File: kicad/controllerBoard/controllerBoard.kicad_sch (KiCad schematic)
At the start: 2 parts, among them J1 Conn_02x20_Top_Bottom, J2 Conn_02x20_Top_Bottom

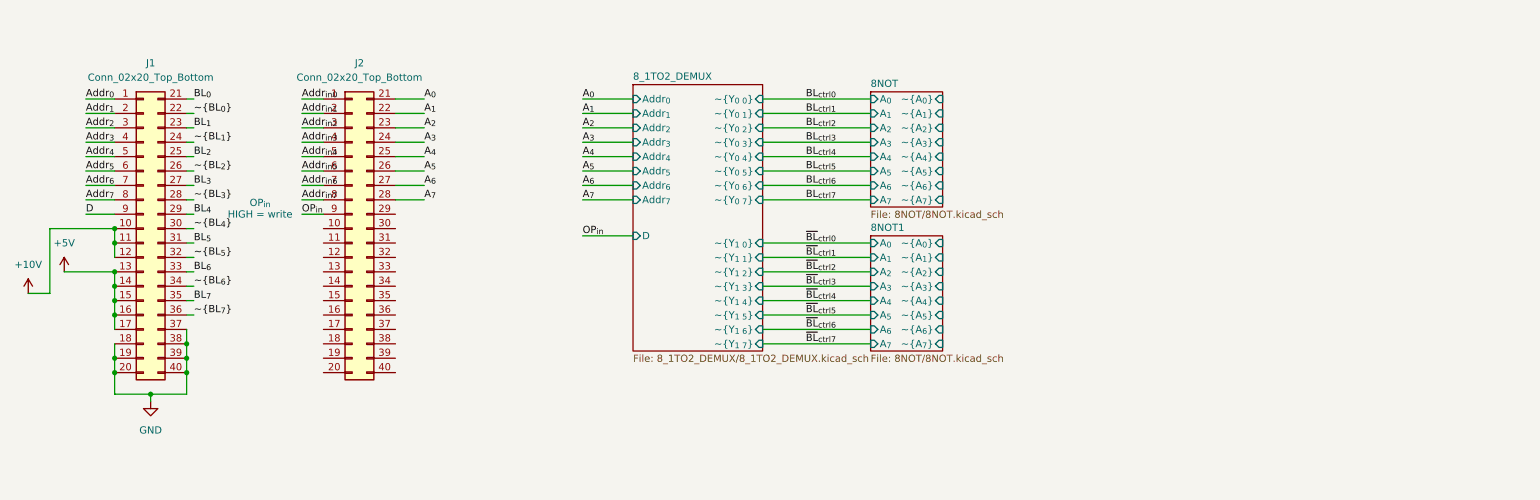
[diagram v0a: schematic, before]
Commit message: demux
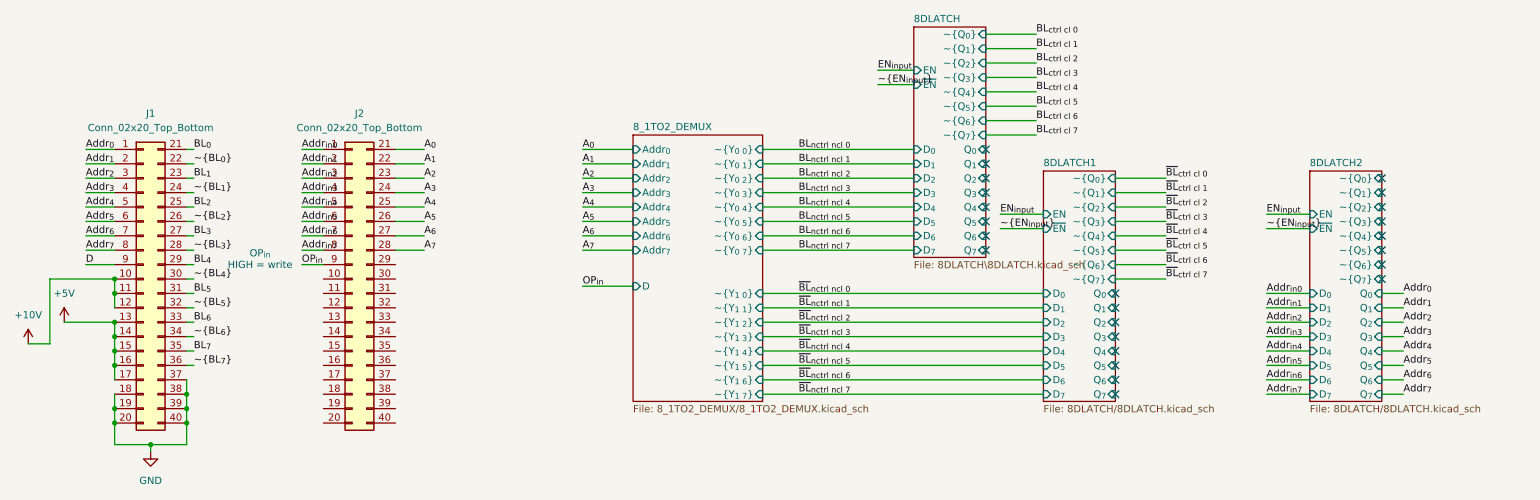
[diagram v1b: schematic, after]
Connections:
- no-connect marks 0 -> 24
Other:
- removed sheet 8NOT
- removed sheet 8NOT1
- added sheet 8DLATCH (8DLATCH\8DLATCH.kicad_sch)
- added sheet 8DLATCH1 (8DLATCH/8DLATCH.kicad_sch)
- added sheet 8DLATCH2 (8DLATCH/8DLATCH.kicad_sch)
- moved on the sheet: J1, J2
